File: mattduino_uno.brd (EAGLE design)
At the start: 68.6 x 53.3 mm, 32 parts, among them IC3 CH340G, IC4 LM317MBSTT3, IC5 NX1117C33Z, J4 POWER_JACK, J6 USB_B_PTH, Q2 16MHz, U1 ATMEGA328P_TQFP, Y1 12Mhz

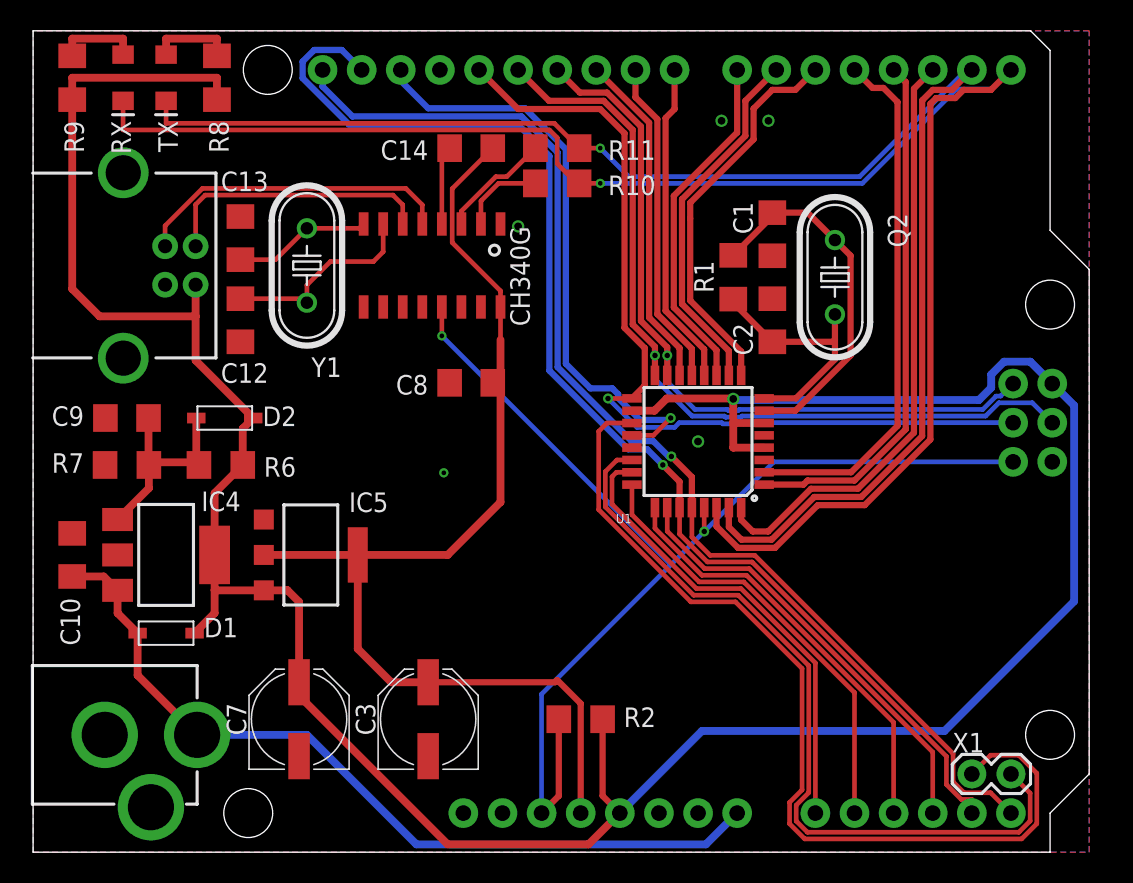
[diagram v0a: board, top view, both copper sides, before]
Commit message: missing stuff
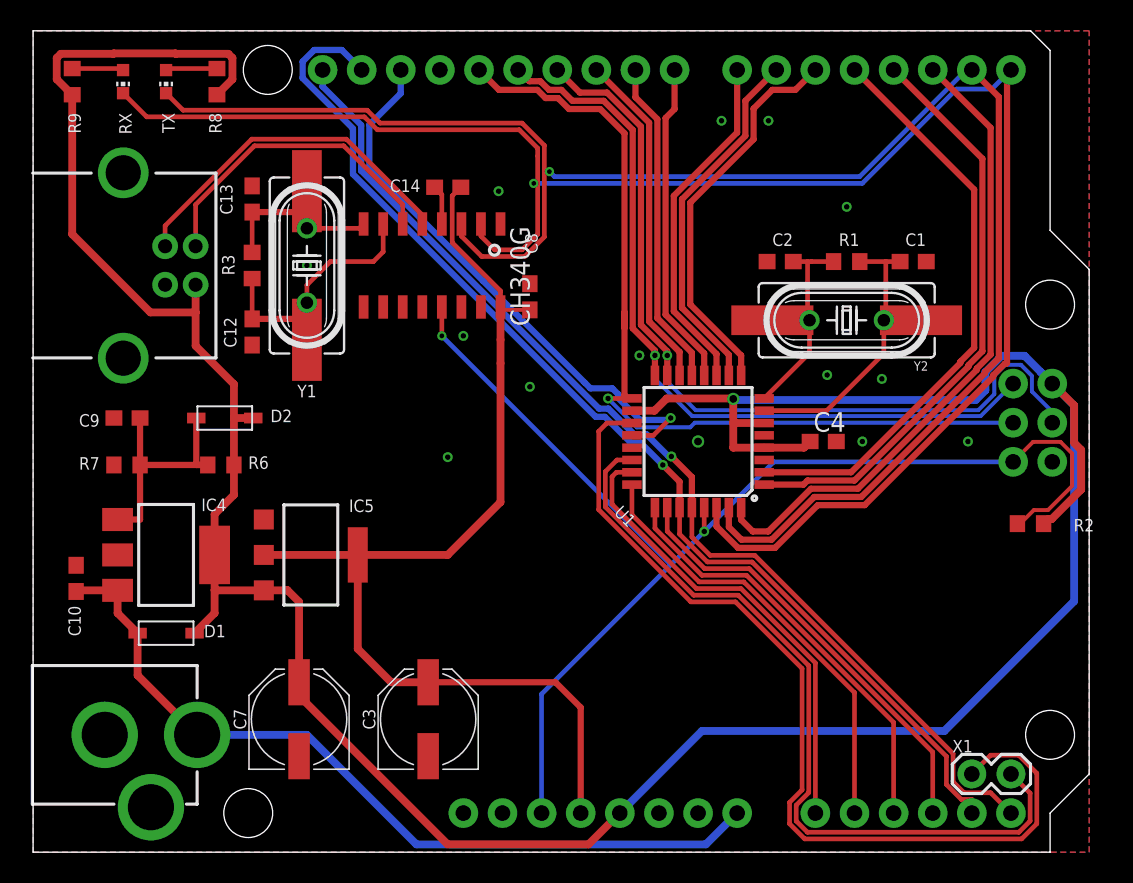
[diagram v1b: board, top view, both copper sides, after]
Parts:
- removed Q2: 16MHz, SparkFun-Clocks:HC49U
- removed R10, R11: 1k, rcl:R1206
- added C4: 0.1uF, rcl:C0603
- added R3: 1M, rcl:R0603
- added Y1B: 12Mhz, SparkFun-Clocks:HC49UP
- added Y2: 16Mhz, SparkFun-Clocks:HC49UP
- added Y2B: 16MHz, SparkFun-Clocks:HC49U
- C1, C10, C12, C13, C14, C2, C8, C9: device rcl:C1206 -> rcl:C0603
- R1, R2, R6, R7, R8, R9: device rcl:R1206 -> rcl:R0603
- RX, TX: device SparkFun-LED:LED-1206 -> led:CHIP-LED0603
- moved R2 31.9 mm to (64.8, 21.3)
- moved C1 9.32 mm to (57.1, 38.4), turned to 0 degrees
- moved R1 7.44 mm to (52.8, 38.4), turned to 180 degrees
- moved C8 6.76 mm to (32.3, 36.1), turned to 90 degrees
- moved C2 3.84 mm to (48.5, 38.4), turned to 180 degrees
- moved C14 2.96 mm to (26.9, 43.2)
- moved C13 2.65 mm to (14.2, 42.4)
- moved C10 1.55 mm to (2.79, 17.8)
- moved C12 1.08 mm to (14.2, 33.8)
- moved R8 0.25 mm to (11.9, 50.0)
- moved R9 0.25 mm to (2.54, 50.0)
- moved RX 0.25 mm to (5.84, 50.0), turned to 180 degrees
- moved TX 0.25 mm to (8.64, 50.0), turned to 180 degrees
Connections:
- net N$3 renamed V3
- removed net CH340_RX: IC3.3, R11.1
- removed net CH340_TX: IC3.2, R10.1
- net +5V: now also C4.1
- net 328_OSC1: now also Y2.1, Y2B.1; no longer Q2.1
- net 328_OSC2: now also Y2.2, Y2B.2; no longer Q2.2
- net GND: now also C4.2
- net IO11/MOSI: now also B2.MOSI; no longer B2.MISO
- net IO12/MISO: now also B2.MISO; no longer B2.MOSI
- net OSCI: now also R3.1, Y1B.1
- net OSCO: now also R3.2, Y1B.2
- net RX: now also IC3.2; no longer R10.2
- net TX: now also IC3.3; no longer R11.2
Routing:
- net TX: track 100.9 -> 113.4 mm
- net +5V: track 190.1 -> 201.6 mm
- net CH340_RX: track 7.33 -> 0.00 mm
- net RX: track 111.6 -> 118.4 mm
- net AD5/SCL: track 76.8 -> 70.4 mm
- net AD4/SDA: track 80.7 -> 74.3 mm
- net IO11/MOSI: track 49.5 -> 55.8 mm
- net CH340_TX: track 5.50 -> 0.00 mm
- net OSCI: track 13.2 -> 18.4 mm
- net RESET: track 75.6 -> 80.4 mm
- net OSCO: track 8.96 -> 13.4 mm
- net IO3: track 34.3 -> 38.5 mm
- net IO4: track 34.6 -> 38.3 mm
- net IO2: track 39.1 -> 42.2 mm
- net USB-: track 17.9 -> 20.6 mm
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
